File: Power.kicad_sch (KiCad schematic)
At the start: 6 parts, among them J201 USB_C_Receptacle_USB2.0, U602 USBLC6-2SC6

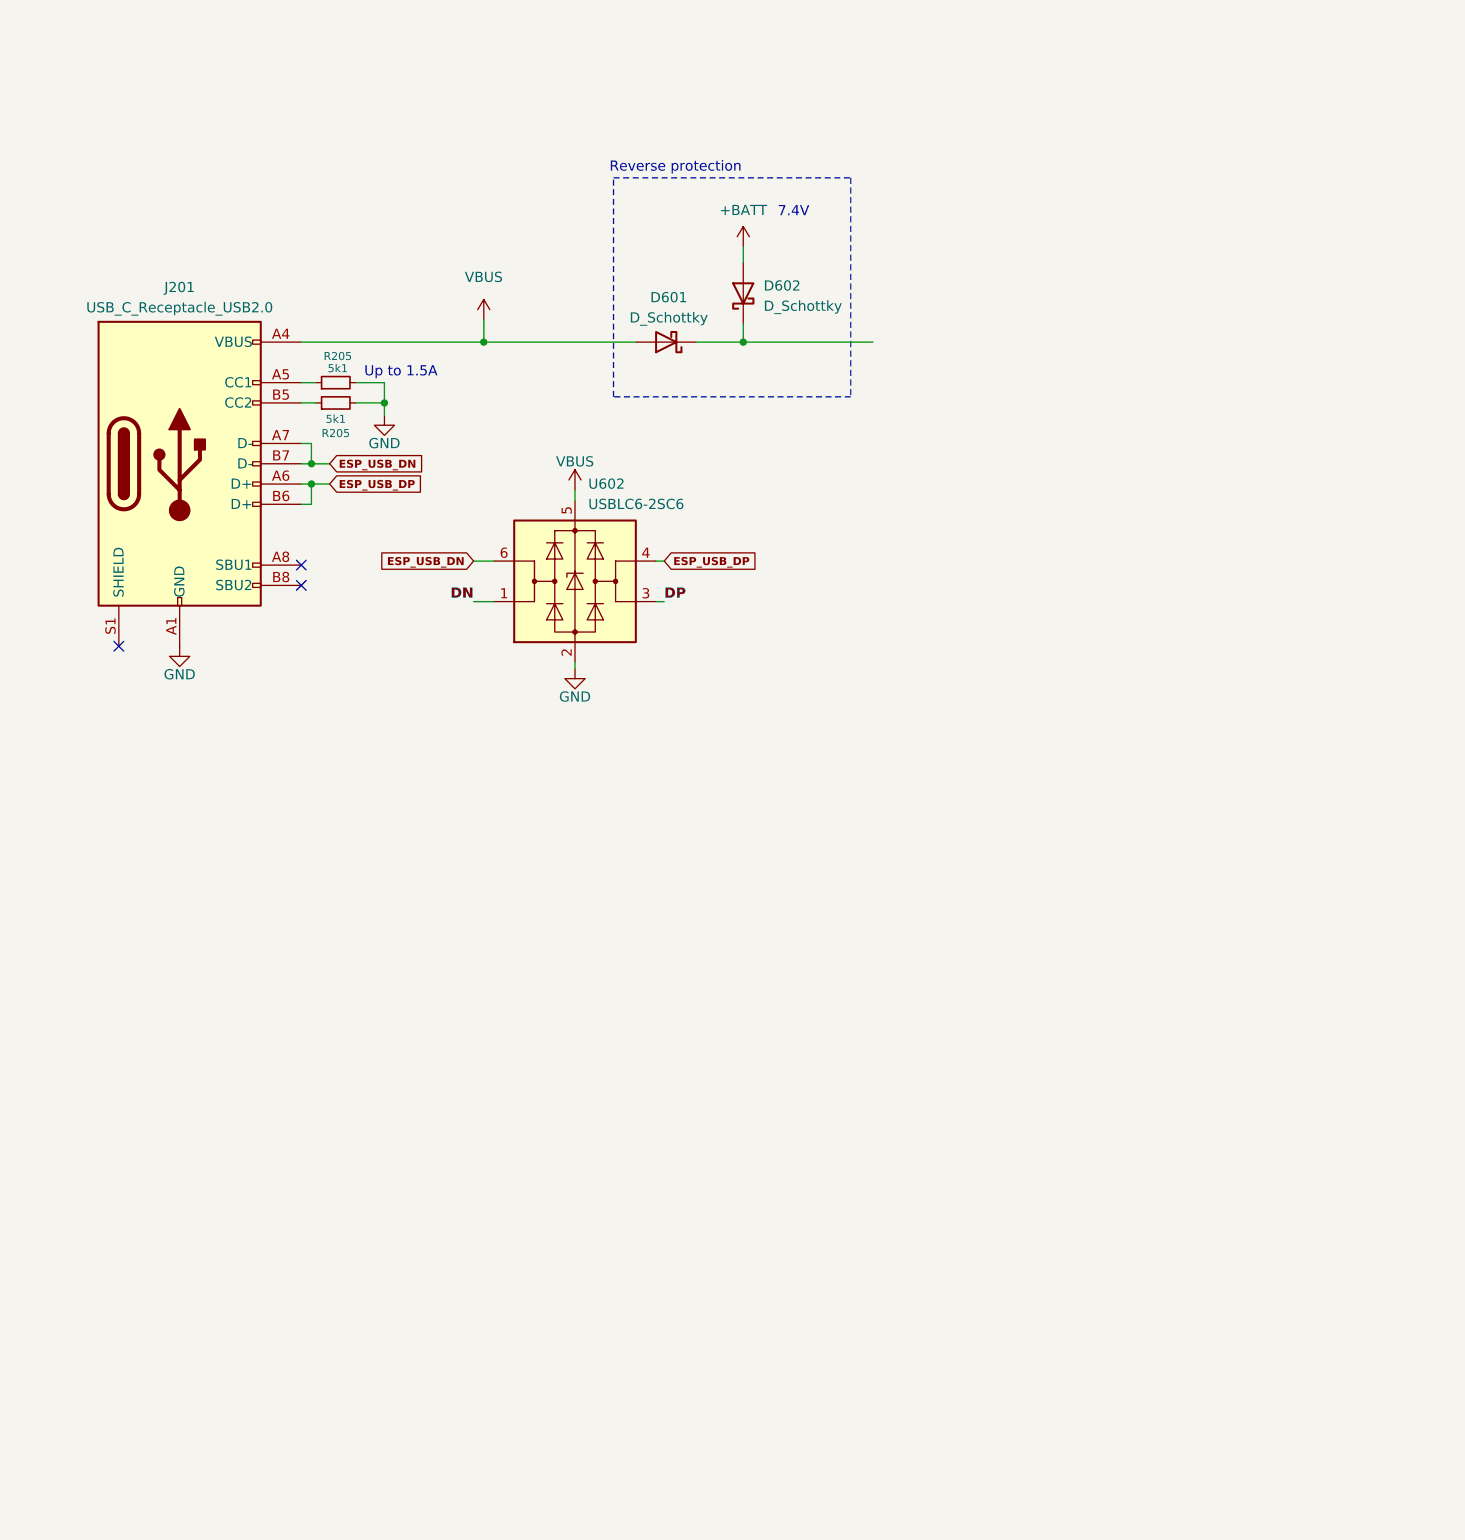
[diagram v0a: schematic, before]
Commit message: trzeba dobrać bucka
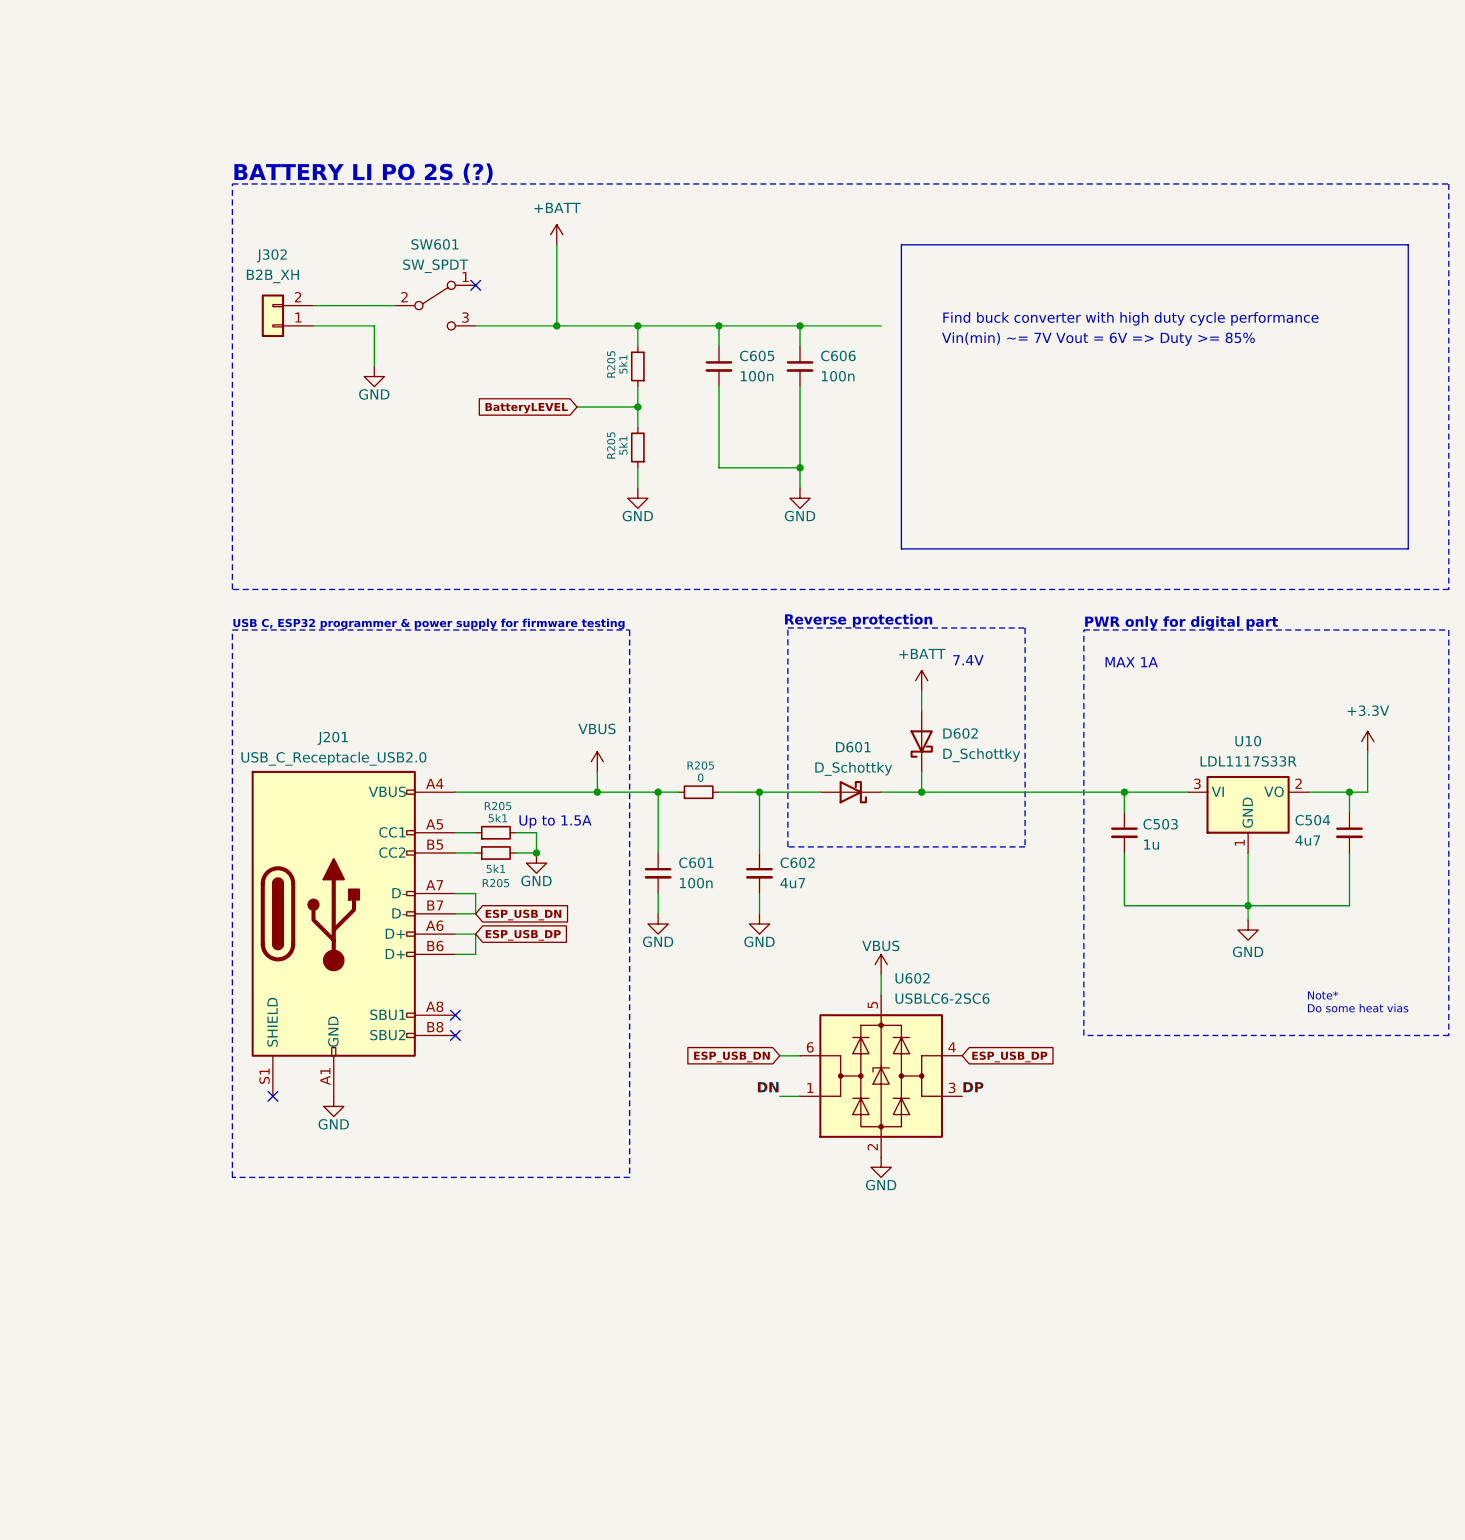
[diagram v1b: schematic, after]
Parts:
- added C503: 1u, Capacitor_SMD:C_0603_1608Metric, symbol Device:C_Small
- added C504: 4u7, Capacitor_SMD:C_0603_1608Metric, symbol Device:C_Small
- added C601, C605, C606: 100n, symbol Device:C_Small
- added C602: 4u7, symbol Device:C_Small
- added J302: B2B_XH, symbol Connector_Generic:Conn_01x02
- added R205 (x2): 5k1, symbol Device:R_Small
- added R205: 0, symbol Device:R_Small
- added SW601: SW_SPDT, symbol Switch:SW_SPDT
- added U10: LDL1117S33R, Package_TO_SOT_SMD:SOT-223-3_TabPin2, symbol Regulator_Linear:LD1117S33TR_SOT223
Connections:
- net +BATT: now also C605.1, C606.1, R205.2, SW601.3 (C)
- net GND: now also C503.2, C504.2, C601.2, C602.2, C605.2, C606.2, J302.1 (Pin_1), R205.1, U10.1 (GND)
- net VBUS: now also C601.1, R205.1; no longer D601.2 (A)
- net at D601.1 (K), D602.1 (K): now also C503.1, U10.3 (VI)
- new net: C602.1, D601.2 (A), R205.2
- new net: J302.2 (Pin_2), SW601.2 (B)
- new net +3.3V: C504.1, U10.2 (VO)
- new net BatteryLEVEL: R205.1, R205.2
- no-connect marks 3 -> 4
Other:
- note added: "BATTERY LI PO 2S (?)"
- note added: "Find buck converter with high duty cycle performance"
- note added: "MAX 1A"
- note added: "Note* Do some heat vias"
- note added: "PWR only for digital part"
- note added: "USB C, ESP32 programmer & power supply for firmware testing"
- note added: "Vin(min) ~= 7V Vout = 6V => Duty >= 85%"
- moved on the sheet: D601, D602, J201, R205, U602

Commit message: Prawie skończone
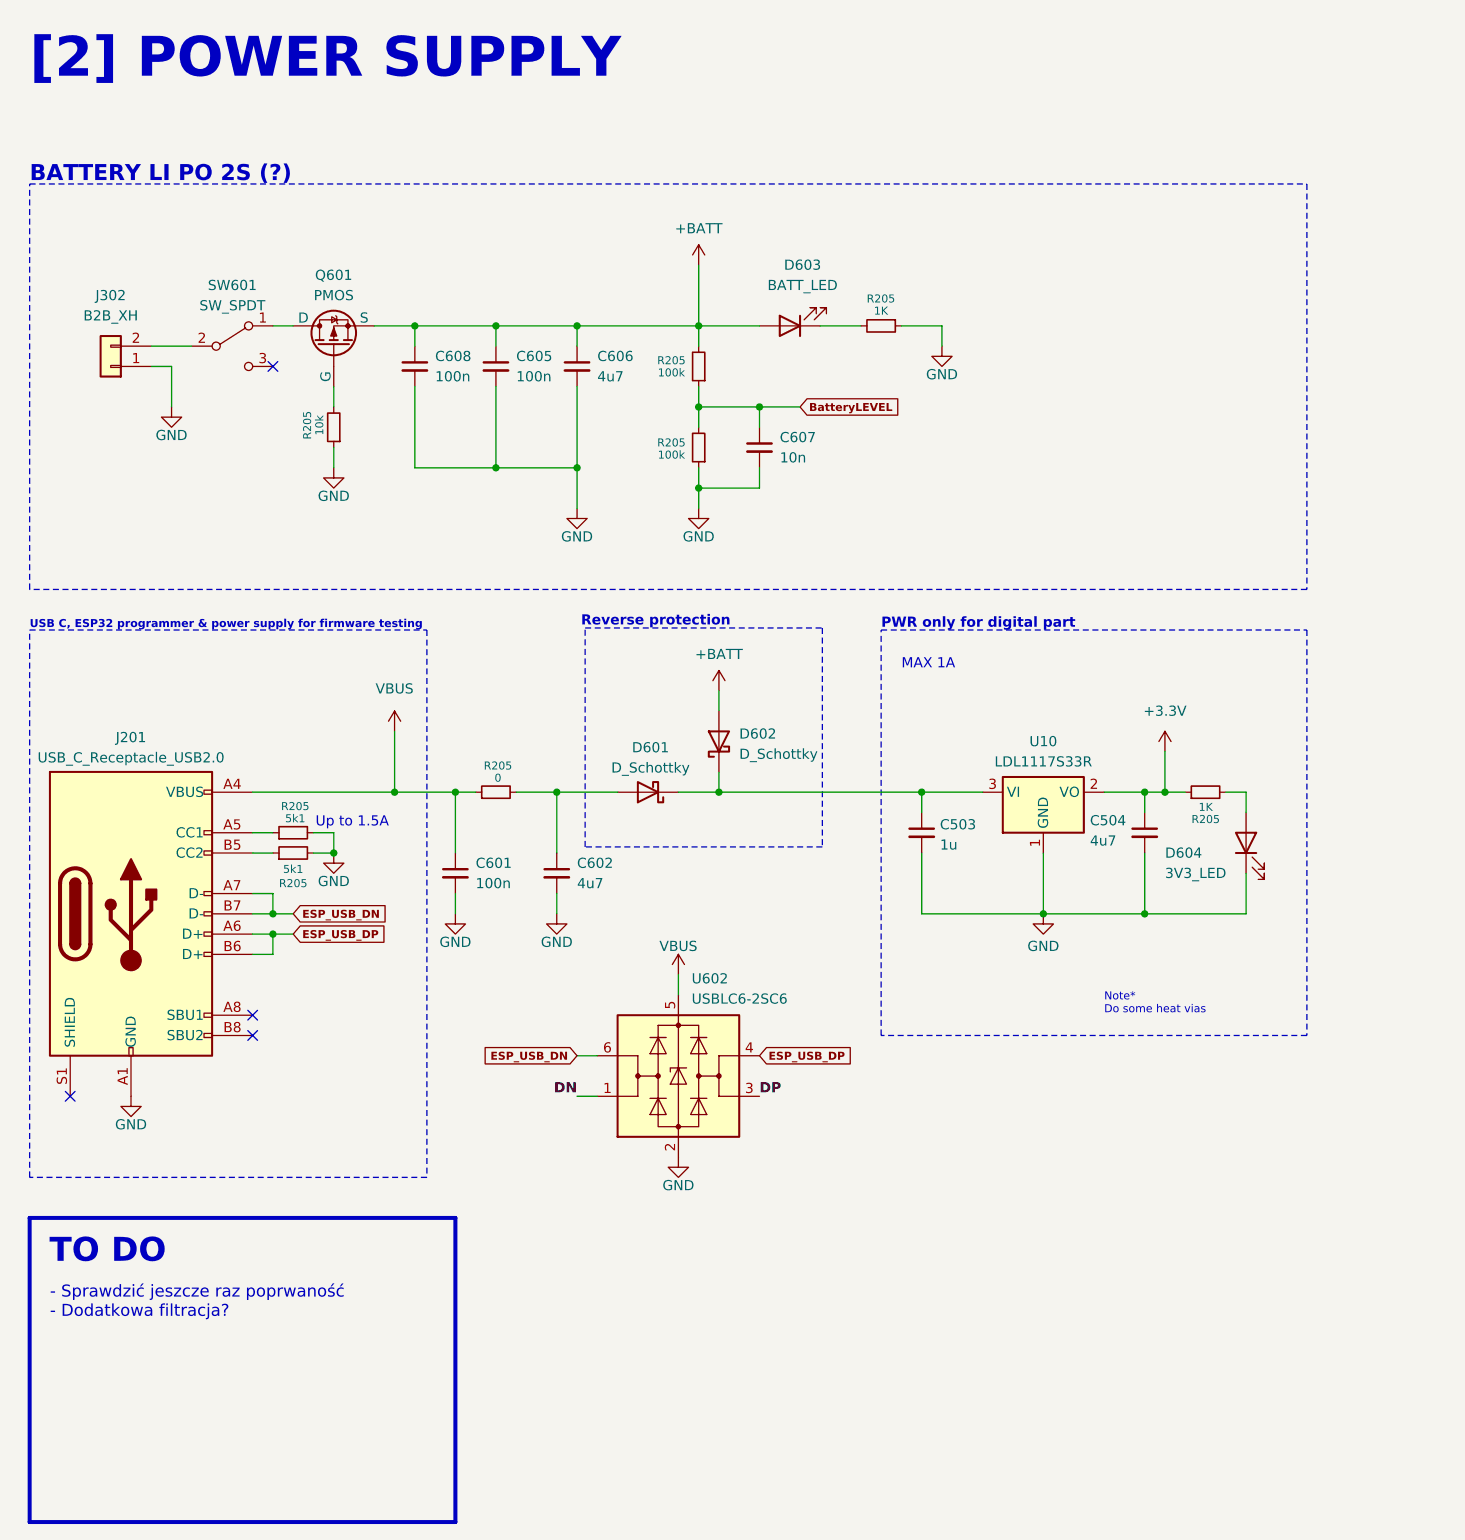
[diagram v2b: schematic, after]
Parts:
- added C607: 10n, symbol Device:C_Small
- added C608: 100n, symbol Device:C_Small
- added D603: BATT_LED, symbol Device:LED
- added D604: 3V3_LED, symbol Device:LED
- added Q601: PMOS, symbol Simulation_SPICE:PMOS
- added R205 (x2): 1K, symbol Device:R_Small
- added R205: 10k, symbol Device:R_Small
- C606: value 100n -> 4u7
- R205: value 5k1 -> 100k
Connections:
- net +3.3V: now also R205.1
- net +BATT: now also C608.1, D603.2 (A), Q601.3 (S); no longer SW601.3 (C)
- net BatteryLEVEL: now also C607.1
- net GND: now also C607.2, C608.2, D604.1 (K), R205.1, R205.1
- net at SW601.1 (A): now also Q601.1 (D)
- new net: D604.2 (A), R205.2
- new net: Q601.2 (G), R205.2
- new net: D603.1 (K), R205.2
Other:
- note added: "- Sprawdzić jeszcze raz poprwaność - Dodatkowa filtracja?"
- note added: "TO DO"
- note added: "[2] POWER SUPPLY"
- note removed: "7.4V"
- note removed: "Find buck converter with high duty cycle performance"
- note removed: "Vin(min) ~= 7V Vout = 6V => Duty >= 85%"
- moved on the sheet: C503, C504, C601, C602, C605, C606, D601, J201, J302, R205, SW601, U10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

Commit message: Dodaje wszystko nie chce mi sie z tym bawic
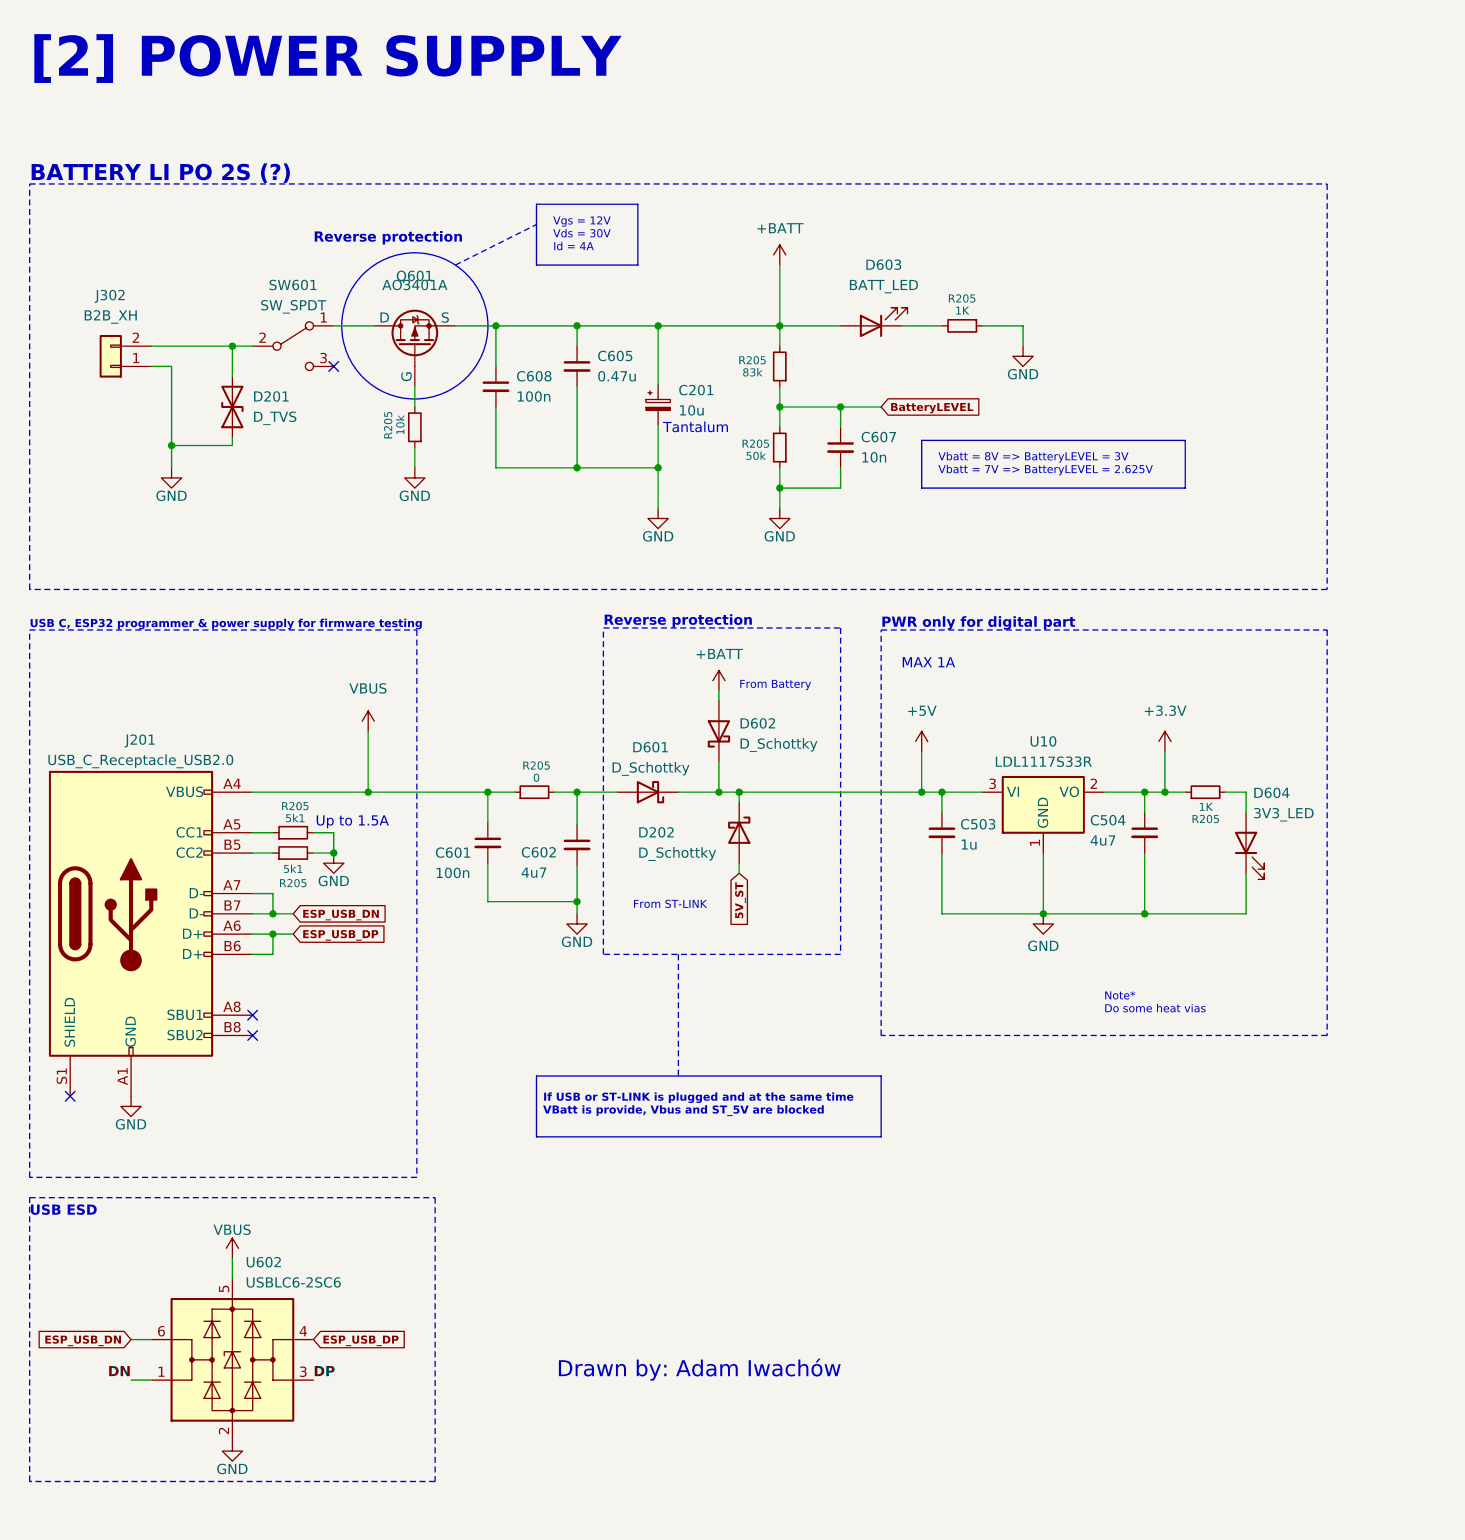
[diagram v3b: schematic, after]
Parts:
- removed C606: 4u7, symbol Device:C_Small
- added C201: 10u, Capacitor_Tantalum_SMD:CP_EIA-3216-10_Kemet-I_Pad1.58x1.35mm_HandSolder, symbol Device:C_Polarized_Small
- added D201: D_TVS, symbol Device:D_TVS
- added D202: D_Schottky, Adam_lib:D_SOD-123FL, symbol Device:D_Schottky
- C601, C602, C607, C608: footprint (none) -> Capacitor_SMD:C_0603_1608Metric
- C605: value 100n -> 0.47u; footprint (none) -> Capacitor_SMD:C_0603_1608Metric
- D601, D602: footprint (none) -> Adam_lib:D_SOD-123FL
- D603, D604: footprint (none) -> LED_SMD:LED_0603_1608Metric
- J302: footprint (none) -> Connector_PinHeader_2.54mm:PinHeader_1x02_P2.54mm_Vertical
- Q601: value PMOS -> AO3401A; footprint (none) -> Package_TO_SOT_SMD:SOT-23-3
- R205: footprint (none) -> Resistor_SMD:R_0603_1608Metric
- R205: value 100k -> 50k; footprint (none) -> Resistor_SMD:R_0603_1608Metric
- R205: value 100k -> 83k; footprint (none) -> Resistor_SMD:R_0603_1608Metric
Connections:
- net +BATT: now also C201.1
- net GND: now also C201.2, D201.1 (A1)
- net +5V: now reaches C503.1, D601.1 (K), D602.1 (K), U10.3 (VI)
- net +5V: now also D202.1 (K)
- net at J302.2 (Pin_2), SW601.2 (B): now also D201.2 (A2)
- new net 5V_ST: D202.2 (A)
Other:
- note added: "Drawn by: Adam Iwachów"
- note added: "From Battery"
- note added: "From ST-LINK"
- note added: "If USB or ST-LINK is plugged and at the same time VBatt is provide, Vbus and ST_5V are blocked"
- note added: "Tantalum"
- note added: "USB ESD"
- note added: "Vbatt = 8V => BatteryLEVEL = 3V Vbatt = 7V => BatteryLEVEL = 2.625V"
- note added: "Vgs = 12V Vds = 30V Id = 4A"
- note removed: "- Sprawdzić jeszcze raz poprwaność - Dodatkowa filtracja?"
- note removed: "TO DO"
- moved on the sheet: C503, C601, C602, C605, C607, C608, D602, D603, Q601, R205, SW601, U602
